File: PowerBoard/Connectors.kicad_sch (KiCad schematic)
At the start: 0 parts

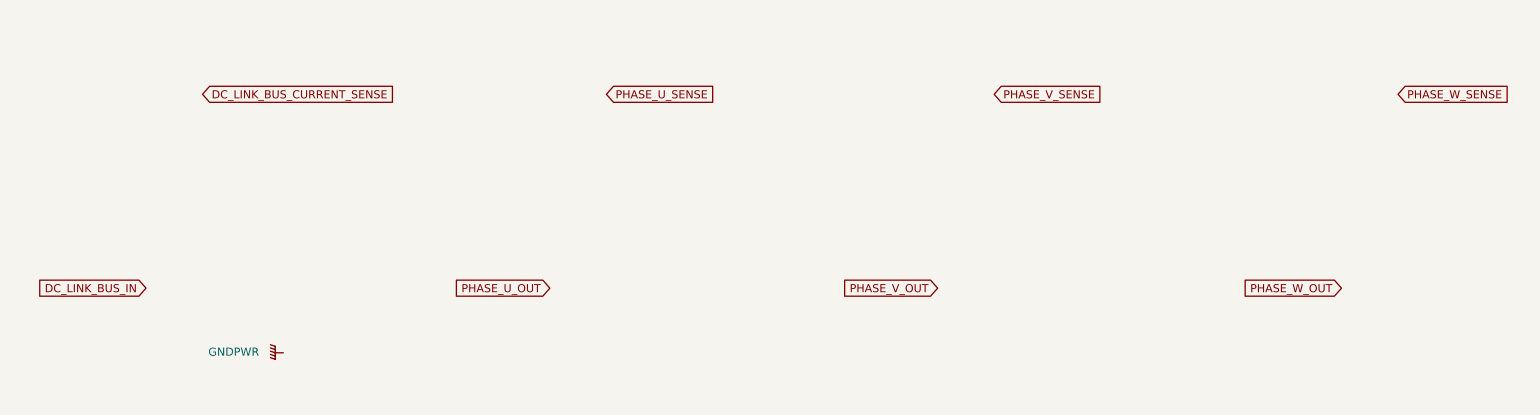
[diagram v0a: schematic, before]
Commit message: u
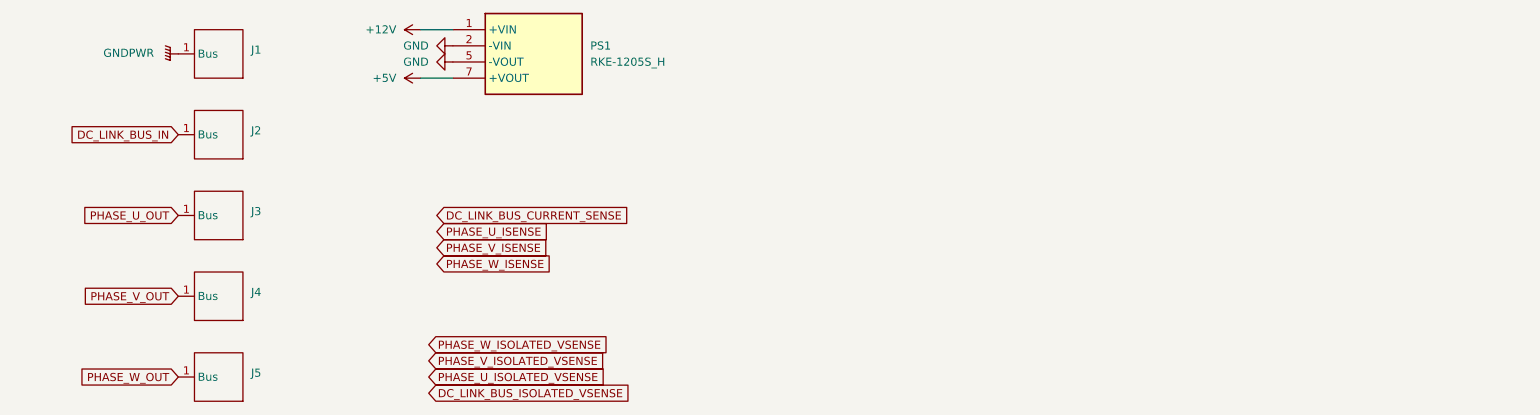
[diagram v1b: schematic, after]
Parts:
- added J1, J2, J3, J4, J5: ~, symbol InverterCom:BusBarConnection
- added PS1: RKE-1205S_H, RKE1205SH, symbol InverterCom:RKE-1205S_H
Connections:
- net DC_LINK_BUS_IN: now also J2.1 (Bus)
- net GNDPWR: now also J1.1 (Bus)
- net PHASE_U_OUT: now also J3.1 (Bus)
- net PHASE_V_OUT: now also J4.1 (Bus)
- net PHASE_W_OUT: now also J5.1 (Bus)
- new net +12V: PS1.1 (+VIN)
- new net +5V: PS1.7 (+VOUT)
- new net GND: PS1.2 (-VIN), PS1.5 (-VOUT)

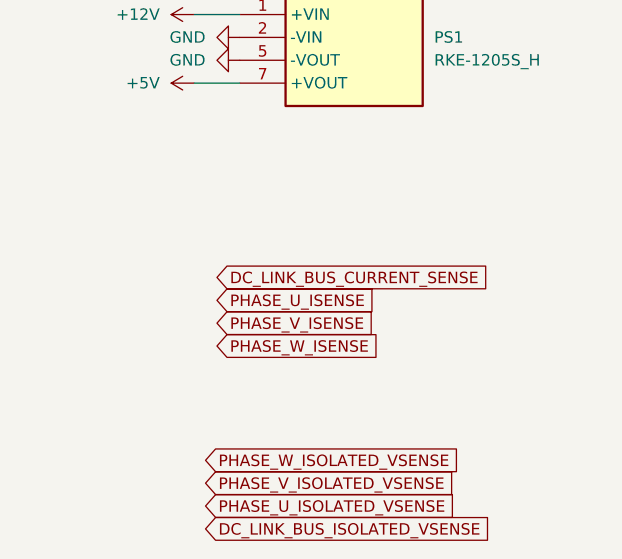
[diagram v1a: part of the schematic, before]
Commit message: vsense
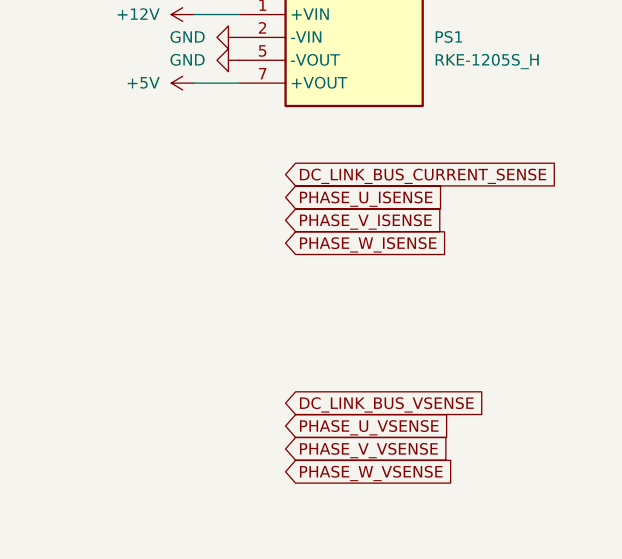
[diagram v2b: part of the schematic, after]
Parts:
- J1, J2, J3, J4, J5: footprint (none) -> InverterCom:BusBarConnection
- PS1: footprint RKE1205SH -> InverterCom:RKE1205SH
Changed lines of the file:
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@@
 		)
 	)
-	(global_label "PHASE_V_ISOLATED_VSENSE"
-		(shape input)
-		(at 77.47 73.66 0)
+	(global_label "PHASE_W_OUT"
+		(shape input)
+		(at 38.1 76.2 180)
+		(fields_autoplaced yes)
+		(effects
+			(font
+				(size 1.27 1.27)
+			)
+			(justify right)
+		)
+		(property "Intersheetrefs" "${INTERSHEET_REFS}"
+			(at 22.052 76.2 0)
+			(effects
+				(font
+					(size 1.27 1.27)
+				)
+				(justify right)
+				(hide yes)
+			)
+		)
+	)
+	(global_label "PHASE_W_ISENSE"
+		(shape input)
+		(at 86.36 46.99 0)
 		(fields_autoplaced yes)
 		(effects
@@
 		)
 		(property "Intersheetrefs" "${INTERSHEET_REFS}"
-			(at 106.2784 73.66 0)
-			(effects
-				(font
-					(size 1.27 1.27)
-				)
-				(justify left)
-				(hide yes)
-			)
-		)
-	)
-	(global_label "PHASE_W_OUT"
-		(shape input)
-		(at 38.1 76.2 180)
+			(at 105.4317 46.99 0)
+			(effects
+				(font
+					(size 1.27 1.27)
+				)
+				(justify left)
+				(hide yes)
+			)
+		)
+	)
+	(global_label "DC_LINK_BUS_CURRENT_SENSE"
+		(shape input)
+		(at 86.36 39.37 0)
+		(fields_autoplaced yes)
+		(effects
+			(font
+				(size 1.27 1.27)
+			)
+			(justify left)
+		)
+		(property "Intersheetrefs" "${INTERSHEET_REFS}"
+			(at 118.4341 39.37 0)
+			(effects
+				(font
+					(size 1.27 1.27)
+				)
+				(justify left)
+				(hide yes)
+			)
+		)
+	)
+	(global_label "PHASE_U_ISENSE"
+		(shape input)
+		(at 86.36 41.91 0)
+		(fields_autoplaced yes)
+		(effects
+			(font
+				(size 1.27 1.27)
+			)
+			(justify left)
+		)
+		(property "Intersheetrefs" "${INTERSHEET_REFS}"
+			(at 105.3108 41.91 0)
+			(effects
+				(font
+					(size 1.27 1.27)
+				)
+				(justify left)
+				(hide yes)
+			)
+		)
+	)
+	(global_label "PHASE_U_VSENSE"
+		(shape input)
+		(at 86.36 67.31 0)
+		(fields_autoplaced yes)
+		(effects
+			(font
+				(size 1.27 1.27)
+			)
+			(justify left)
+		)
+		(property "Intersheetrefs" "${INTERSHEET_REFS}"
+			(at 105.7946 67.31 0)
+			(effects
+				(font
+					(size 1.27 1.27)
+				)
+				(justify left)
+				(hide yes)
+			)
+		)
+	)
+	(global_label "PHASE_U_OUT"
+		(shape input)
+		(at 38.1 50.8 180)
 		(fields_autoplaced yes)
 		(effects
@@
 		)
 		(property "Intersheetrefs" "${INTERSHEET_REFS}"
-			(at 22.052 76.2 0)
-			(effects
-				(font
-					(size 1.27 1.27)
-				)
-				(justify right)
-				(hide yes)
-			)
-		)
-	)
-	(global_label "PHASE_W_ISOLATED_VSENSE"
-		(shape input)
-		(at 77.47 71.12 0)
+			(at 22.1729 50.8 0)
+			(effects
+				(font
+					(size 1.27 1.27)
+				)
+				(justify right)
+				(hide yes)
+			)
+		)
+	)
+	(global_label "PHASE_V_ISENSE"
+		(shape input)
+		(at 86.36 44.45 0)
 		(fields_autoplaced yes)
 		(effects
@@
 		)
 		(property "Intersheetrefs" "${INTERSHEET_REFS}"
-			(at 106.6412 71.12 0)
-			(effects
-				(font
-					(size 1.27 1.27)
-				)
-				(justify left)
-				(hide yes)
-			)
-		)
-	)
-	(global_label "PHASE_W_ISENSE"
-		(shape input)
-		(at 78.74 58.42 0)
+			(at 105.0689 44.45 0)
+			(effects
+				(font
+					(size 1.27 1.27)
+				)
+				(justify left)
+				(hide yes)
+			)
+		)
+	)
+	(global_label "PHASE_W_VSENSE"
+		(shape input)
+		(at 86.36 72.39 0)
 		(fields_autoplaced yes)
 		(effects
@@
 		)
 		(property "Intersheetrefs" "${INTERSHEET_REFS}"
-			(at 97.8117 58.42 0)
-			(effects
-				(font
-					(size 1.27 1.27)
-				)
-				(justify left)
-				(hide yes)
-			)
-		)
-	)
-	(global_label "DC_LINK_BUS_ISOLATED_VSENSE"
-		(shape input)
-		(at 77.47 78.74 0)
+			(at 105.9155 72.39 0)
+			(effects
+				(font
+					(size 1.27 1.27)
+				)
+				(justify left)
+				(hide yes)
+			)
+		)
+	)
+	(global_label "PHASE_V_VSENSE"
+		(shape input)
+		(at 86.36 69.85 0)
 		(fields_autoplaced yes)
 		(effects
@@
 		)
 		(property "Intersheetrefs" "${INTERSHEET_REFS}"
-			(at 110.6932 78.74 0)
-			(effects
-				(font
-					(size 1.27 1.27)
-				)
-				(justify left)
-				(hide yes)
-			)
-		)
-	)
-	(global_label "DC_LINK_BUS_CURRENT_SENSE"
-		(shape input)
-		(at 78.74 50.8 0)
+			(at 105.5527 69.85 0)
+			(effects
+				(font
+					(size 1.27 1.27)
+				)
+				(justify left)
+				(hide yes)
+			)
+		)
+	)
+	(global_label "DC_LINK_BUS_VSENSE"
+		(shape input)
+		(at 86.36 64.77 0)
 		(fields_autoplaced yes)
 		(effects
@@
 		)
 		(property "Intersheetrefs" "${INTERSHEET_REFS}"
-			(at 110.8141 50.8 0)
-			(effects
-				(font
-					(size 1.27 1.27)
-				)
-				(justify left)
-				(hide yes)
-			)
-		)
-	)
-	(global_label "PHASE_U_ISENSE"
-		(shape input)
-		(at 78.74 53.34 0)
-		(fields_autoplaced yes)
-		(effects
-			(font
-				(size 1.27 1.27)
-			)
-			(justify left)
-		)
-		(property "Intersheetrefs" "${INTERSHEET_REFS}"
-			(at 97.6908 53.34 0)
-			(effects
-				(font
-					(size 1.27 1.27)
-				)
-				(justify left)
-				(hide yes)
-			)
-		)
-	)
-	(global_label "PHASE_U_OUT"
-		(shape input)
-		(at 38.1 50.8 180)
-		(fields_autoplaced yes)
-		(effects
-			(font
-				(size 1.27 1.27)
-			)
-			(justify right)
-		)
-		(property "Intersheetrefs" "${INTERSHEET_REFS}"
-			(at 22.1729 50.8 0)
-			(effects
-				(font
-					(size 1.27 1.27)
-				)
-				(justify right)
-				(hide yes)
-			)
-		)
-	)
-	(global_label "PHASE_V_ISENSE"
-		(shape input)
-		(at 78.74 55.88 0)
-		(fields_autoplaced yes)
-		(effects
-			(font
-				(size 1.27 1.27)
-			)
-			(justify left)
-		)
-		(property "Intersheetrefs" "${INTERSHEET_REFS}"
-			(at 97.4489 55.88 0)
-			(effects
-				(font
-					(size 1.27 1.27)
-				)
-				(justify left)
-				(hide yes)
-			)
-		)
-	)
-	(global_label "PHASE_U_ISOLATED_VSENSE"
-		(shape input)
-		(at 77.47 76.2 0)
-		(fields_autoplaced yes)
-		(effects
-			(font
-				(size 1.27 1.27)
-			)
-			(justify left)
-		)
-		(property "Intersheetrefs" "${INTERSHEET_REFS}"
-			(at 106.5203 76.2 0)
+			(at 109.9675 64.77 0)
 			(effects
 				(font
@@
 			)
 		)
-		(property "Footprint" ""
+		(property "Footprint" "InverterCom:BusBarConnection"
 			(at 45.212 54.356 0)
 			(effects
@@
 			)
 		)
-		(property "Footprint" "RKE1205SH"
+		(property "Footprint" "InverterCom:RKE1205SH"
 			(at 102.87 116.51 0)
 			(effects
@@
 			)
 		)
-		(property "Footprint" ""
+		(property "Footprint" "InverterCom:BusBarConnection"
 			(at 45.212 67.056 0)
 			(effects
@@
 			)
 		)
-		(property "Footprint" ""
+		(property "Footprint" "InverterCom:BusBarConnection"
 			(at 45.212 41.656 0)
 			(effects
@@
 			)
 		)
-		(property "Footprint" ""
+		(property "Footprint" "InverterCom:BusBarConnection"
 			(at 45.212 79.756 0)
 			(effects
@@
 			)
 		)
-		(property "Footprint" ""
+		(property "Footprint" "InverterCom:BusBarConnection"
 			(at 45.212 28.956 0)
 			(effects

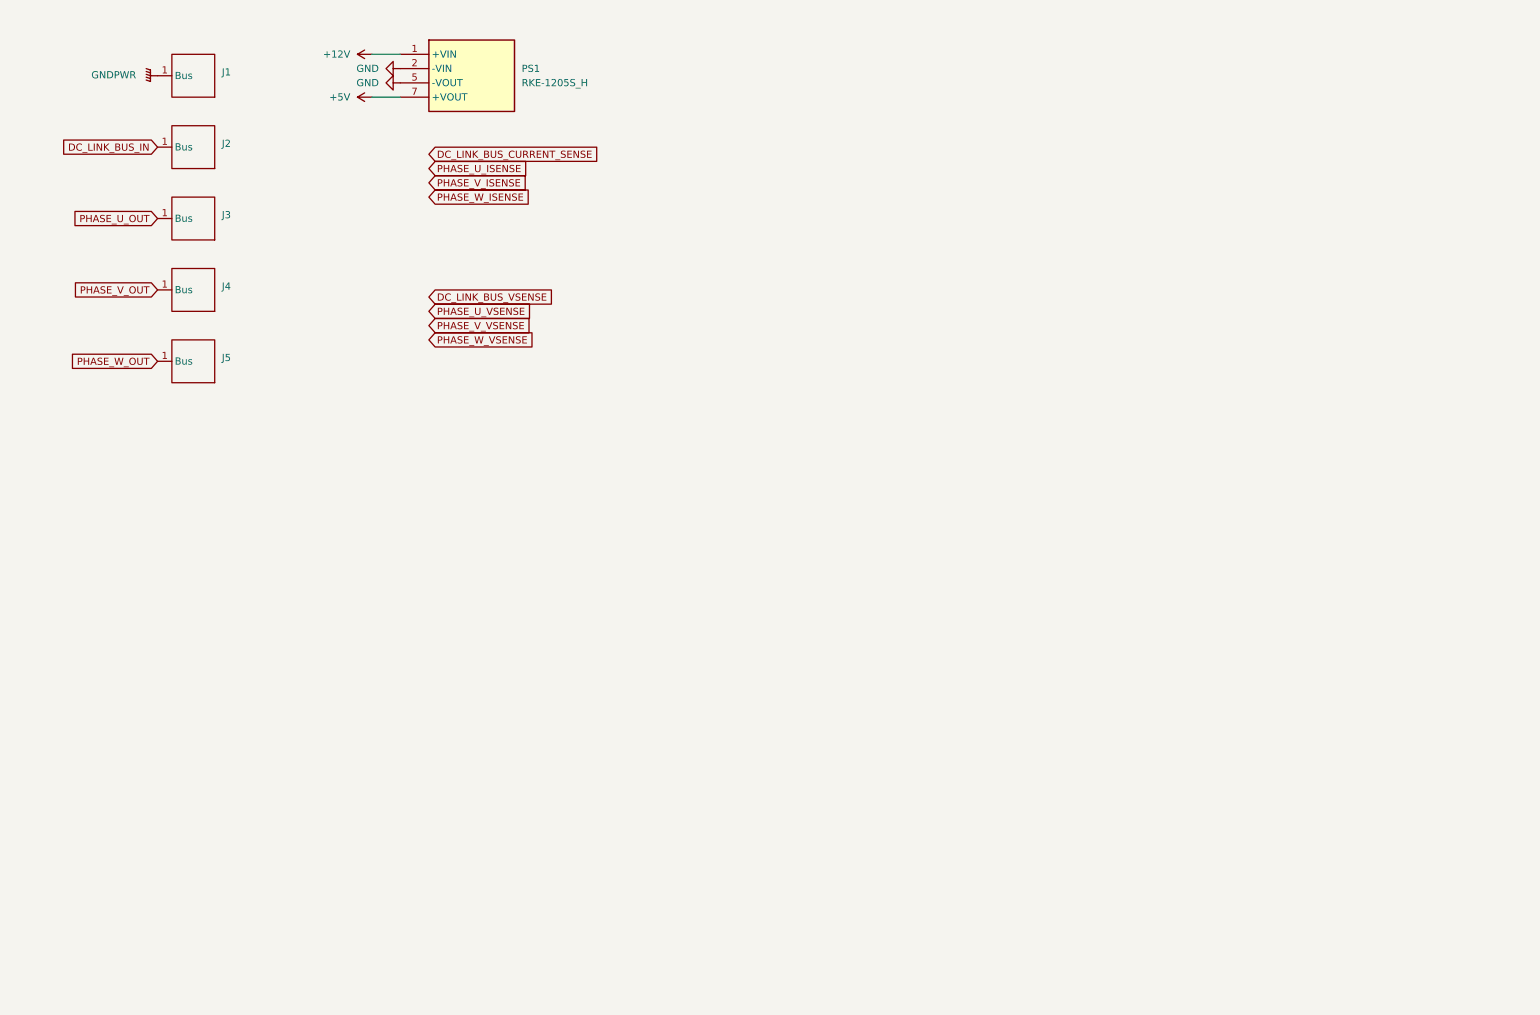
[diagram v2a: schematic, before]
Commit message: Update
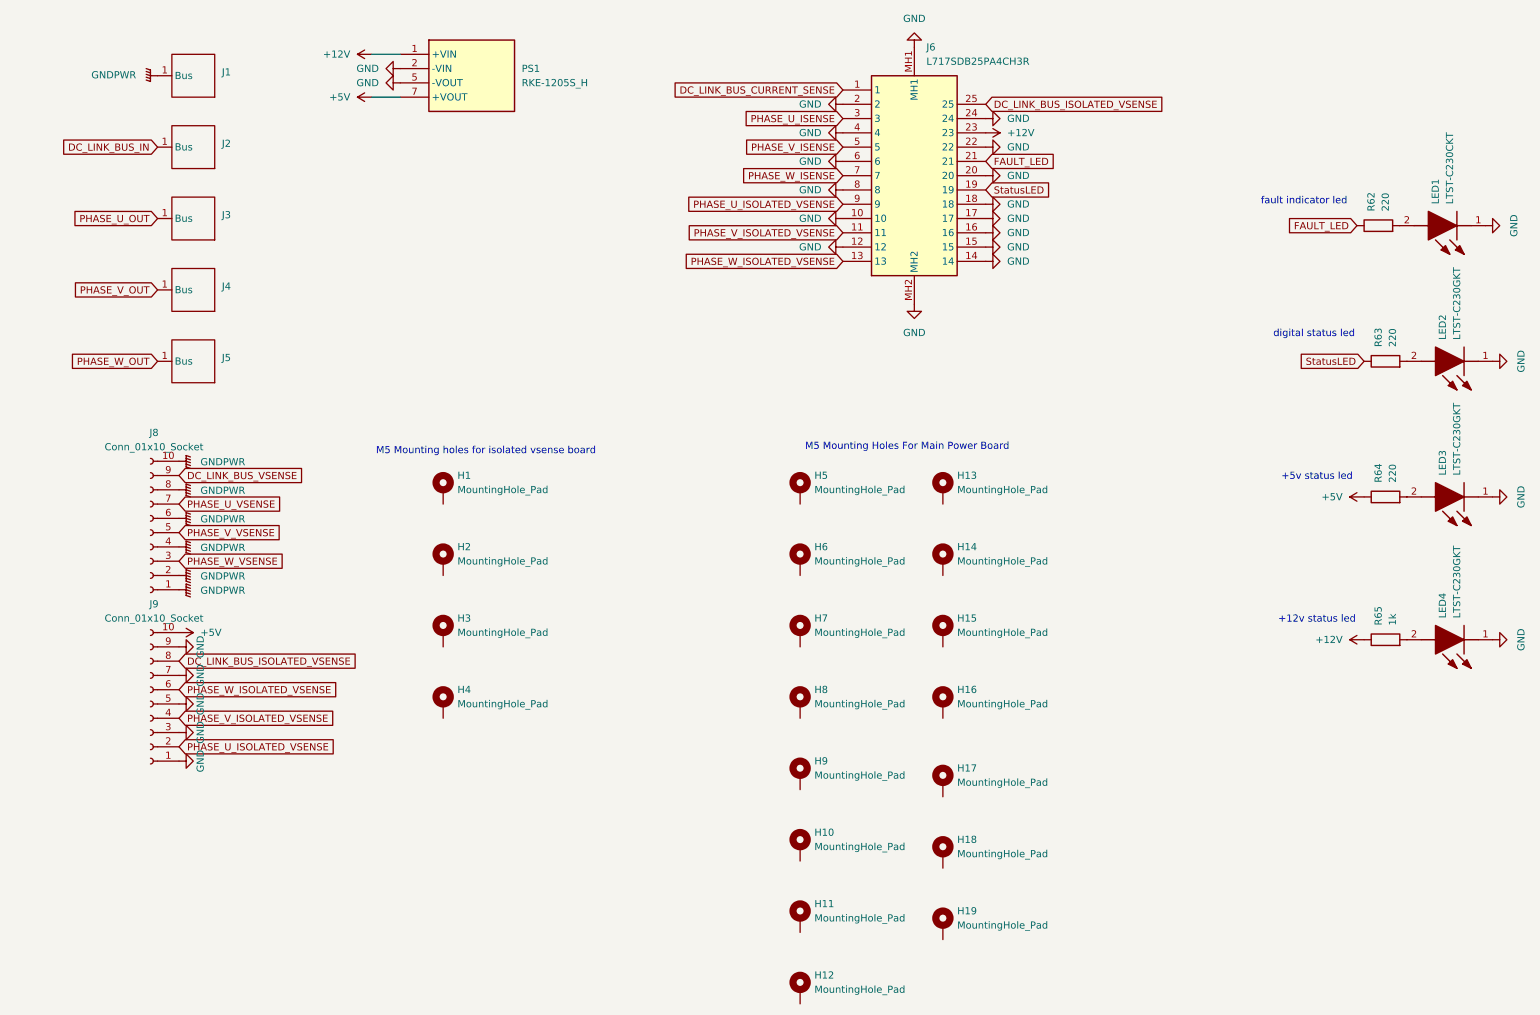
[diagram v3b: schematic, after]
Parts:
- added H1, H10, H11, H12, H13, H14, H15, H16, H17, H18, H19, H2, H3, H4, H5, H6, H7, H8, H9: MountingHole_Pad, MountingHole:MountingHole_5.3mm_M5_ISO7380_Pad, symbol Mechanical:MountingHole_Pad
- added J6: L717SDB25PA4CH3R, InverterCom:L717SDB25PA4CH3R, symbol InverterCom:L717SDB25PA4CH3R
- added J8, J9: Conn_01x10_Socket, Connector_PinSocket_2.54mm:PinSocket_1x10_P2.54mm_Vertical, symbol Connector:Conn_01x10_Socket
- added LED1: LTST-C230CKT, InverterCom:LEDC3216X120N, symbol InverterCom:LTST-C230CKT
- added LED2, LED3, LED4: LTST-C230GKT, InverterCom:LEDC3216X120N, symbol InverterCom:LTST-C230GKT
- added R62, R63, R64: 220, Resistor_SMD:R_1210_3225Metric_Pad1.30x2.65mm_HandSolder, symbol Device:R
- added R65: 1k, Resistor_SMD:R_1210_3225Metric_Pad1.30x2.65mm_HandSolder, symbol Device:R
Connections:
- net +12V: now also J6.23, R65.1
- net +5V: now also J9.10 (Pin_10), R64.1
- net DC_LINK_BUS_CURRENT_SENSE: now also J6.1
- net DC_LINK_BUS_VSENSE: now also J8.9 (Pin_9)
- net GND: now also J6.10, J6.12, J6.14, J6.15, J6.16, J6.17, J6.18, J6.2, J6.20, J6.22, J6.24, J6.4, J6.6, J6.8, J6.MH1, J6.MH2, J9.1 (Pin_1), J9.3 (Pin_3), J9.5 (Pin_5), J9.7 (Pin_7), J9.9 (Pin_9), LED1.1 (K), LED2.1 (K), LED3.1 (K), LED4.1 (K)
- net GNDPWR: now also J8.1 (Pin_1), J8.10 (Pin_10), J8.2 (Pin_2), J8.4 (Pin_4), J8.6 (Pin_6), J8.8 (Pin_8)
- net PHASE_U_ISENSE: now also J6.3
- net PHASE_U_VSENSE: now also J8.7 (Pin_7)
- net PHASE_V_ISENSE: now also J6.5
- net PHASE_V_VSENSE: now also J8.5 (Pin_5)
- net PHASE_W_ISENSE: now also J6.7
- net PHASE_W_VSENSE: now also J8.3 (Pin_3)
- new net: LED3.2 (A), R64.2
- new net: LED4.2 (A), R65.2
- new net: LED1.2 (A), R62.2
- new net: LED2.2 (A), R63.2
- new net DC_LINK_BUS_ISOLATED_VSENSE: J6.25, J9.8 (Pin_8)
- new net FAULT_LED: J6.21, R62.1
- new net PHASE_U_ISOLATED_VSENSE: J6.9, J9.2 (Pin_2)
- new net PHASE_V_ISOLATED_VSENSE: J6.11, J9.4 (Pin_4)
- new net PHASE_W_ISOLATED_VSENSE: J6.13, J9.6 (Pin_6)
- new net StatusLED: J6.19, R63.1
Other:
- note added: "+12v status led"
- note added: "+5v status led"
- note added: "M5 Mounting Holes For Main Power Board"
- note added: "M5 Mounting holes for isolated vsense board"
- note added: "digital status led"
- note added: "fault indicator led"
